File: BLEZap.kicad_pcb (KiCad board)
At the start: 2 copper layers, 38.1 x 22.9 mm, 12 parts, among them P1 PRG_HEADER, P2 INPUT_HEADER, P3 CONN_01X02, Q1 IRLML6344, U1 Core51822B

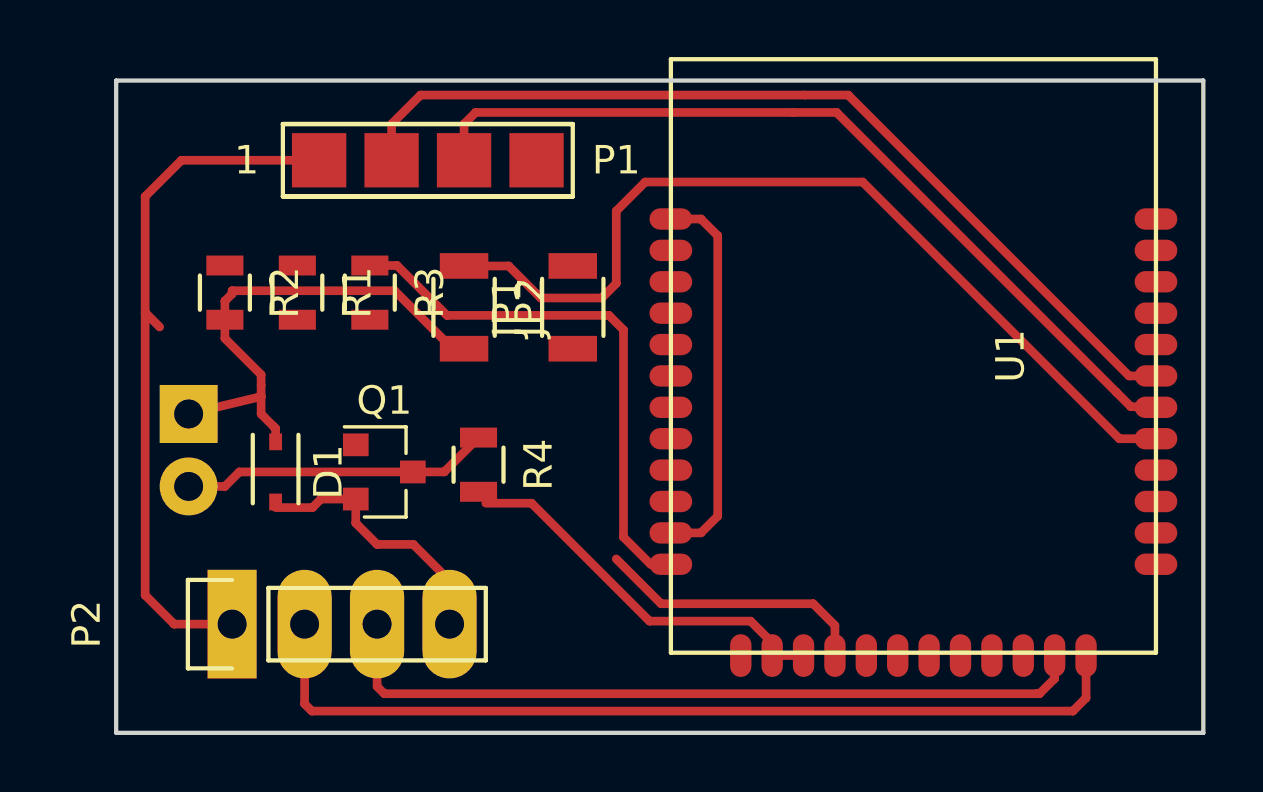
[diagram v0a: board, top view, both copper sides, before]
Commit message: PCB Ready
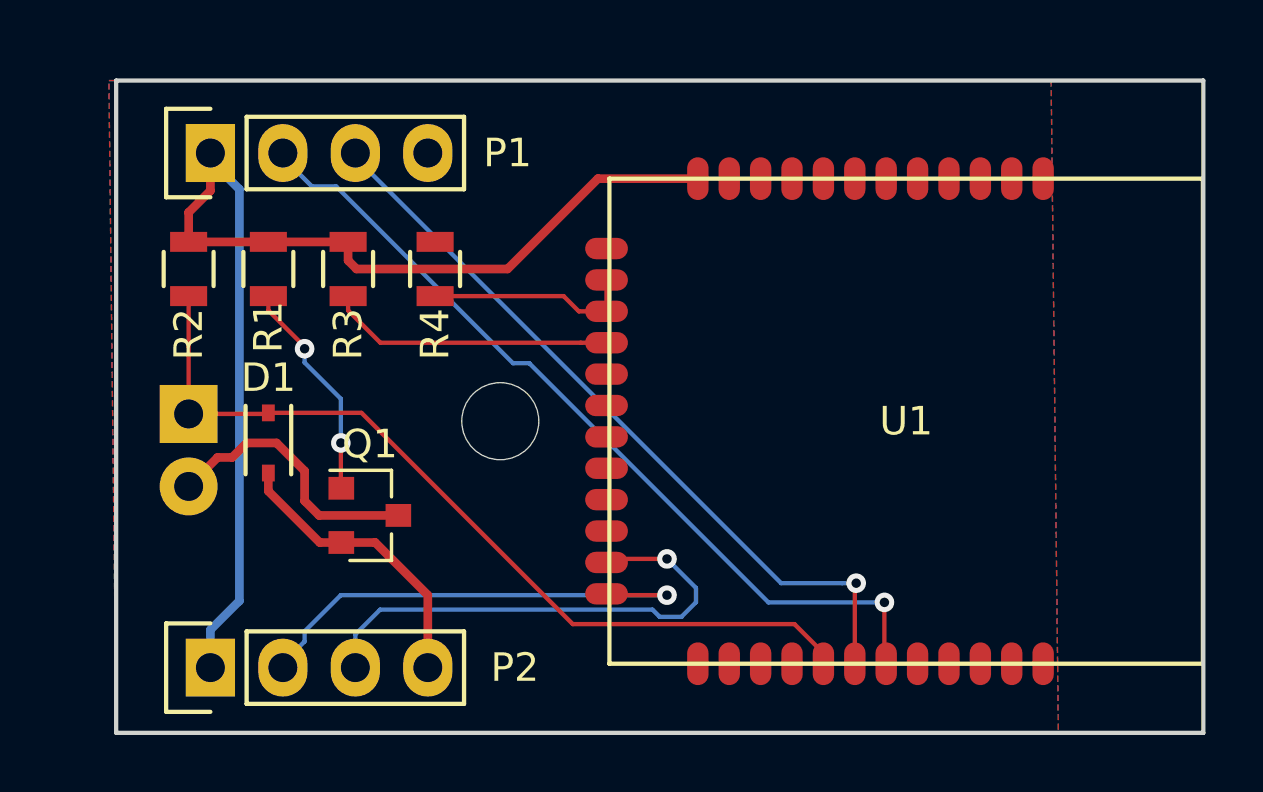
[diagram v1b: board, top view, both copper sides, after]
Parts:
- removed JP1, JP2: Jumper, Resistors_SMD:R_1206
- added REF**: MountingHole_2.7mm_M2.5, Mounting_Holes:MountingHole_2.7mm_M2.5, F.Cu at (89.7, 88.1)
- P1: footprint KevinLibrary:POGO_PIN_PAD_1X4 -> Pin_Headers:Pin_Header_Straight_1x04
- P2: footprint KevinLibrary:Pin_Header_Straight_1x04_HB -> Pin_Headers:Pin_Header_Straight_1x04
- moved P1 7.62 mm to (79.5, 78.7), turned to 90 degrees
- moved R4 7.03 mm to (87.4, 82.8)
- moved U1 2.30 mm to (103.9, 88.1), turned to 0 degrees
- moved P2 1.70 mm to (79.5, 96.8)
- moved Q1 1.61 mm to (85.1, 91.4)
- moved R2 1.52 mm to (78.7, 82.8)
- moved R1 1.31 mm to (81.5, 82.8)
- moved R3 1.13 mm to (84.3, 82.8)
- moved D1 1.05 mm to (81.5, 88.9)
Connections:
- P3 pad 1: Net-(JP2-Pad2) -> Net-(D1-Pad1)
- R2 pad 2: Net-(JP2-Pad2) -> Net-(D1-Pad1)
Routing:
- net Net-(JP2-Pad2): track 16.5 -> 0.00 mm
- net /RELAY: track 32.0 -> 16.9 mm, vias 0 -> 1
- net GNDD: track 24.5 -> 9.65 mm
- net /CFG_BTN: track 27.1 -> 17.9 mm, vias 0 -> 1
- net Net-(Q1-Pad1): track 0.00 -> 7.79 mm, vias 0 -> 2
- net Net-(R4-Pad2): track 13.6 -> 7.33 mm
- net /SWDIO: track 30.0 -> 26.7 mm, vias 0 -> 1
- net GND: track 13.2 -> 10.3 mm
- net /SWCLK: track 32.6 -> 29.9 mm, vias 0 -> 1
- net Net-(D1-Pad1): track 32.6 -> 30.3 mm
- net VDD: track 43.9 -> 42.5 mm
- added copper zone on B.Cu, net GNDD
- added copper zone on F.Cu, net GNDD
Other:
- net class Default: clearance 0.3048 -> 0.254; trace_width 0.3048 -> 0.1524; via_dia 2.54 -> 0.6858; via_drill 0.8382 -> 0.3302
- net class Power added: clearance 0.3048, trace_width 0.3048, via_dia 0.6858, via_drill 0.3302
- rule trace_clearance: 0.3048 -> 0.254
- rule trace_min: 0.3048 -> 0.1524
- rule via_min_drill: 0.8382 -> 0.3302
- rule via_min_size: 2.54 -> 0.6858
